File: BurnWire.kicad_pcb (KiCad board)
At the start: 2 copper layers, 44.6 x 45.4 mm, 14 parts, among them J1 B6B-XH-A_LF__SN_, U1 ADP2303ARDZ

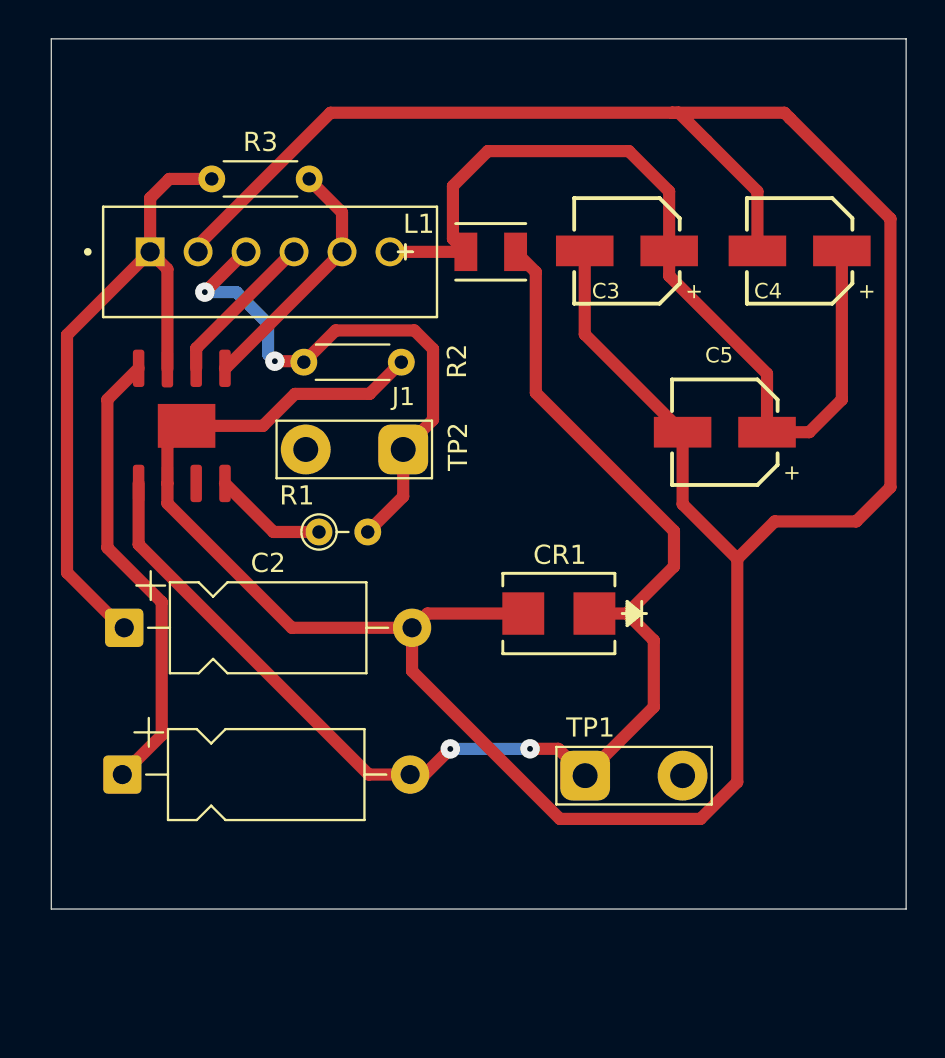
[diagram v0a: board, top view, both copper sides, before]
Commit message: redid layout
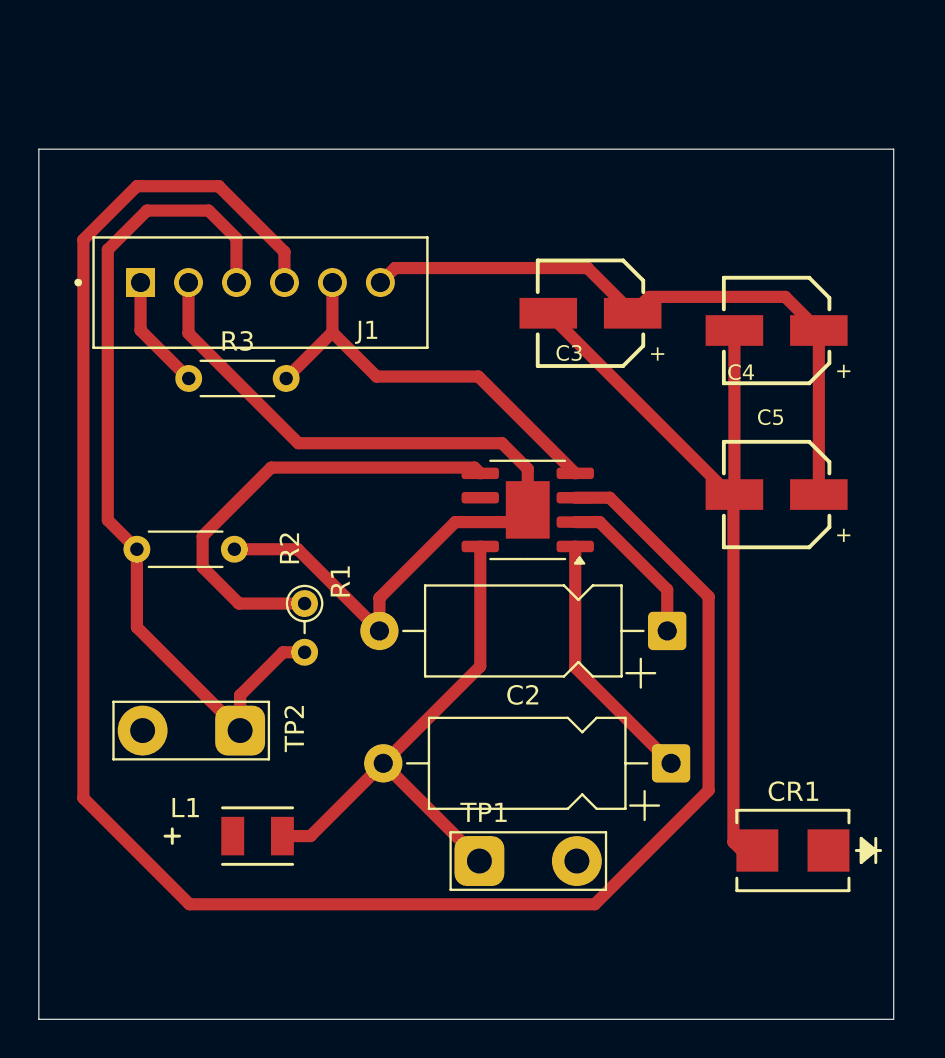
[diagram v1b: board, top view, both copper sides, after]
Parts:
- moved L1 32.8 mm to (141.5, 109.7)
- moved C1 28.6 mm to (163.1, 105.9), turned to 180 degrees
- moved C2 28.3 mm to (162.8, 99.0), turned to 180 degrees
- moved U1 18.3 mm to (155.6, 92.7), turned to 180 degrees
- moved CR1 17.4 mm to (169.4, 110.4)
- moved TP2 16.9 mm to (140.6, 104.2)
- moved R2 13.1 mm to (135.2, 94.7)
- moved R3 10.5 mm to (137.9, 85.8)
- moved TP1 7.08 mm to (153.1, 111.0)
- moved C4 4.32 mm to (168.6, 83.3)
- moved C5 4.23 mm to (168.6, 91.8)
- moved R1 3.80 mm to (143.9, 97.5), turned to -90 degrees
- moved C3 3.76 mm to (158.8, 82.4)
- moved J1 1.68 mm to (141.7, 81.3)
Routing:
- net /EN: track 8.22 -> 100.3 mm
- net GND: track 167.7 -> 87.8 mm
- net Net-(U1-SW): track 68.0 -> 27.4 mm, vias 2 -> 0
- net /VBatt: track 35.6 -> 14.4 mm
- net Net-(U1-FB): track 5.95 -> 23.8 mm
- net /VCutN: track 29.4 -> 44.5 mm, vias 2 -> 0
- net /Vout: track 47.6 -> 33.8 mm
- net Net-(U1-BST): track 23.9 -> 13.4 mm
- net Net-(U1-PGOOD): track 13.1 -> 21.7 mm
